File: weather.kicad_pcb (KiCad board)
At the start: 2 copper layers, 24.1 x 24.1 mm, 23 parts, among them J1 Tag-Connect, U1 nRF52810-QCxx, U2 HDC2080, Y1 32MHz, Y2 32kHz

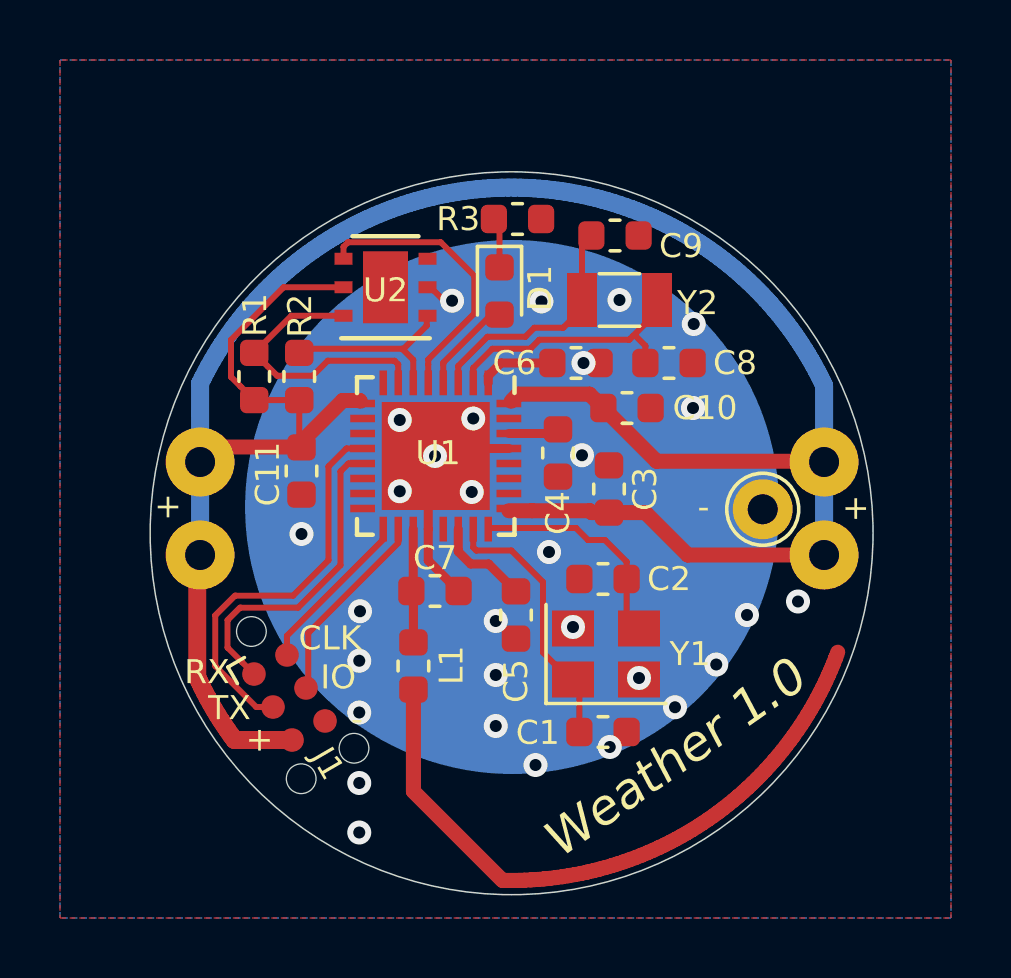
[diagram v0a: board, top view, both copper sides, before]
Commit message: KiCad upgrade
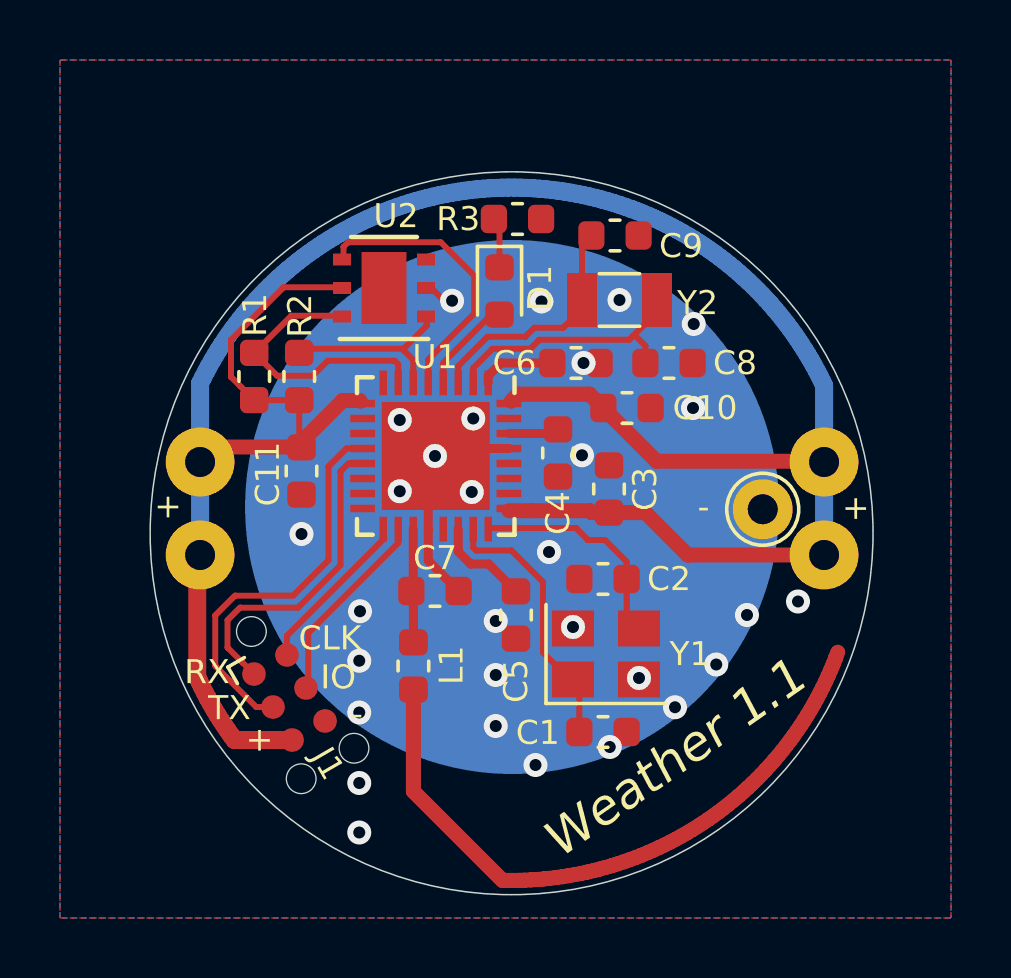
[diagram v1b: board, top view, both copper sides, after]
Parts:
- moved U2 0.06 mm to (107.9, 68.9)
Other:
- board text added: "Weather 1.1"
- board text removed: "Weather 1.0"
